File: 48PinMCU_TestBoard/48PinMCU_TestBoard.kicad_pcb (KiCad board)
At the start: 2 copper layers, 112.1 x 57.3 mm, 111 parts, among them IC1 74LVC1G157GW,125, IC2 TCAN3413DR, J1 USB_C_Receptacle_USB2.0_16P, J2 CAN_Nanofit, J3 Conn_01x03, J5 SWD, J6 USB_C_Receptacle_USB2.0_16P, J7 Conn_01x17, J8 Conn_01x17, SW1 Reset, SW2 SW_SPDT, SW3 BOOT Switch, SW4 RESET Button, U1 STM32G431CBT6, U2 ESP32-C6-MINI-1, U3 MCP1826S, U4 TPS2117DRLR, Y1 Crystal

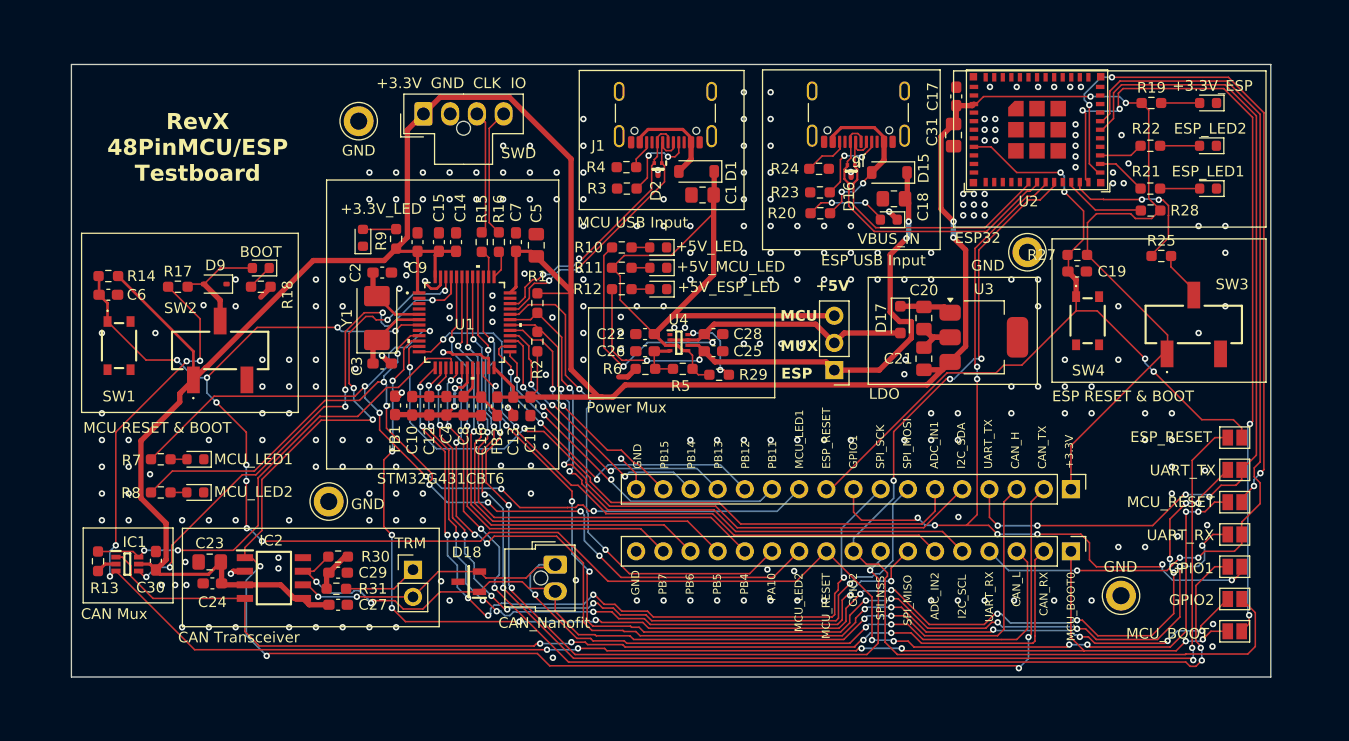
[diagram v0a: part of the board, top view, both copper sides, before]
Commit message: layout tweaks
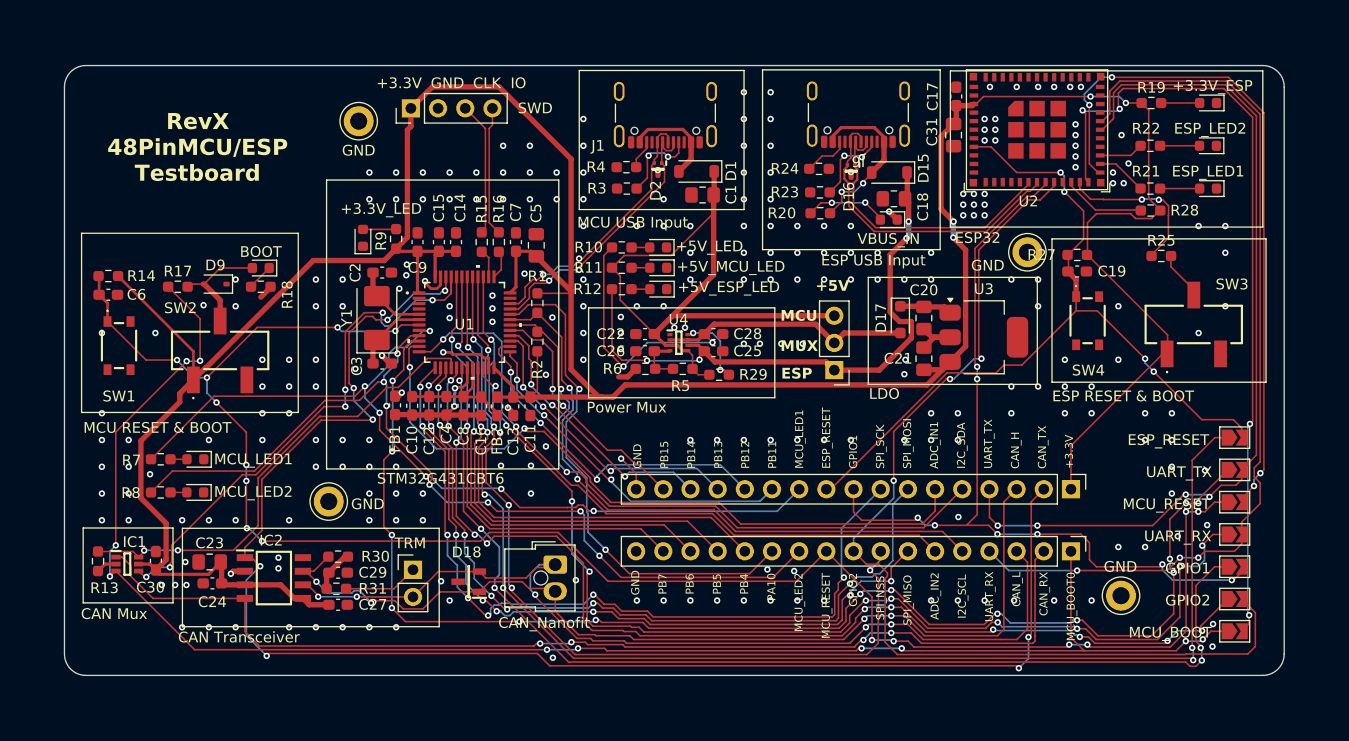
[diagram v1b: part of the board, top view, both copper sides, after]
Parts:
- removed J5: SWD, UTSVT_Connectors:Molex_Nano-Fit_105309-xx04_1x04_P2.50mm_Vertical
- added J4: SWD, Connector_PinHeader_2.54mm:PinHeader_1x04_P2.54mm_Vertical, F.Cu at (111.4, 64.0)
- JP10, JP11, JP12, JP13, JP14, JP8, JP9: footprint Jumper:SolderJumper-2_P1.3mm_Open_Pad1.0x1.5mm -> Jumper:SolderJumper-2_P1.3mm_Open_TrianglePad1.0x1.5mm
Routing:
- net +3.3V: track 308.6 -> 310.4 mm
- net Net-(J4-Pin_3): track 11.1 -> 12.0 mm
- net /I2C_SDA: track 58.1 -> 59.0 mm
- net /PA10: track 47.1 -> 47.8 mm
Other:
- board size 112.1 x 57.3 mm -> 114 x 57 mm
